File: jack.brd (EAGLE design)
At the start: 100 x 80 mm, 30 parts, among them IC1 NUF2221W1T2G, IC2 ATSAMD21G18, IC3 LDO, SW1 SPST3.5X6MM, X1 TSX-3225 24.0000MF10Z-C3

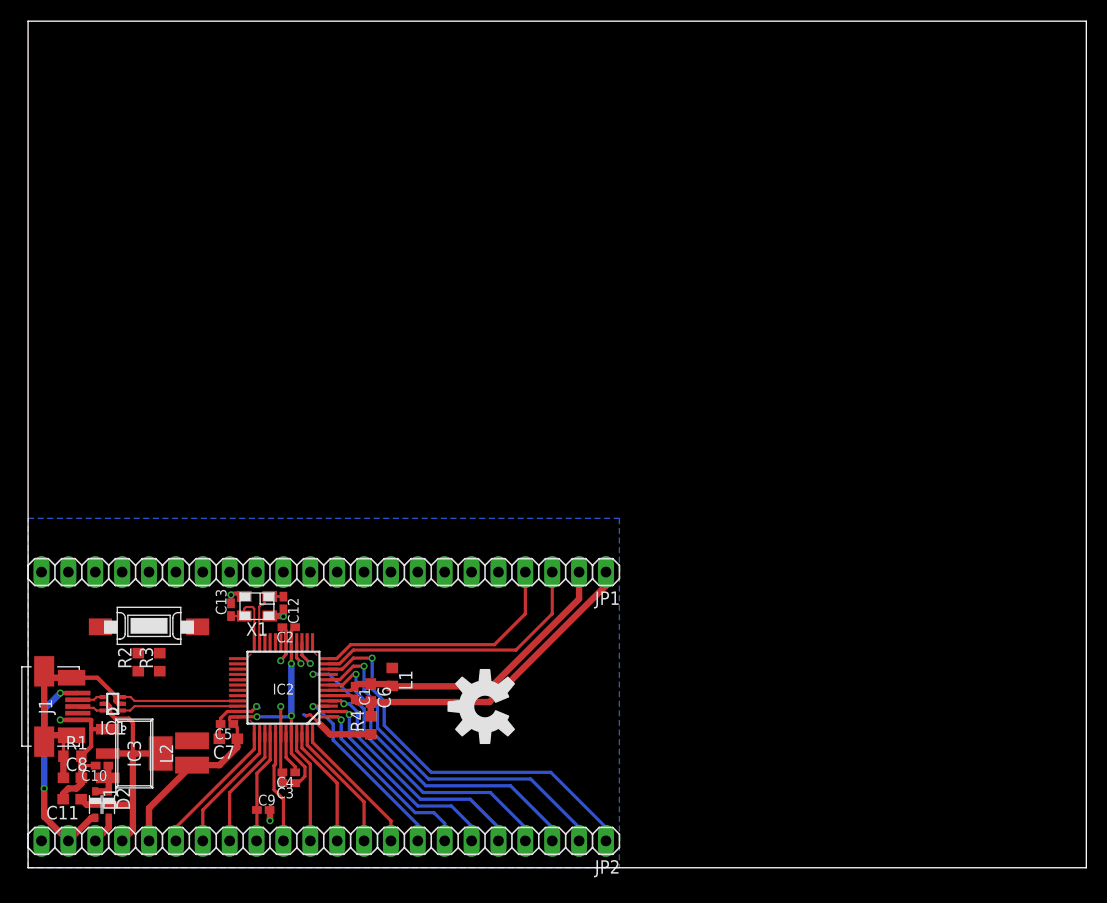
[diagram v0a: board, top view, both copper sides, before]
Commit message: :feelsgood: Layout finished!
Minor details gotta be worked now (polishing pours layout)
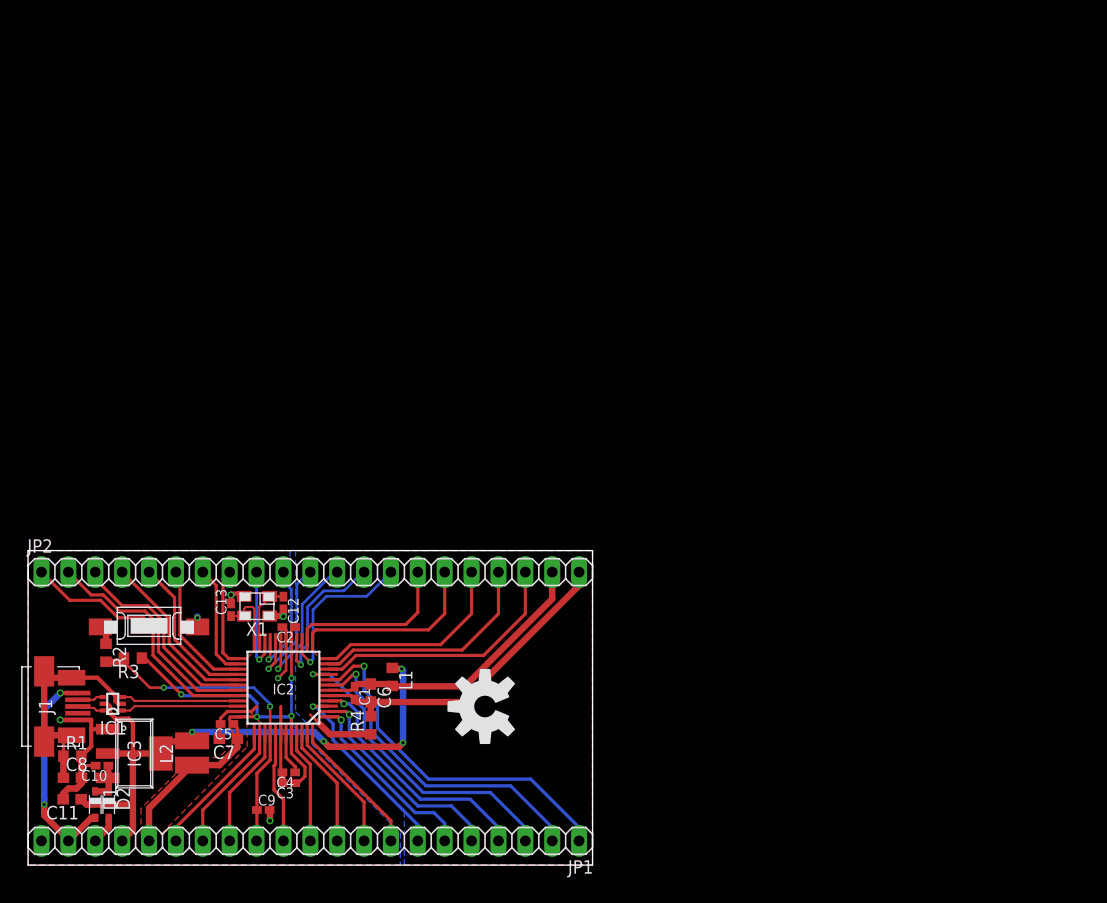
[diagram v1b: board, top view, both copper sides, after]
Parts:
- JP1, JP2: value (none) -> PINHD-1X21; device pinhead:1X22 -> jack:1X21
- moved JP1 25.4 mm to (26.7, 2.54)
- moved JP2 25.4 mm to (26.7, 27.9), turned to 0 degrees
- moved R2 3.18 mm to (7.37, 20.3), turned to 270 degrees
- moved R3 2.57 mm to (9.91, 19.8), turned to 180 degrees
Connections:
- removed net NC: JP1.10, JP1.11, JP1.12, JP1.13, JP1.14, JP1.15, JP1.16, JP1.17, JP1.18, JP1.9
- net !RESET: now also JP1.13; no longer JP2.14
- net 1: now also JP1.6; no longer JP2.7
- net 10: now also JP2.19; no longer JP2.1
- net 11: now also JP2.18; no longer JP1.3
- net 12: now also JP2.17; no longer JP1.4
- net 13: now also JP2.16; no longer JP1.5
- net 14: now also JP2.15; no longer JP1.6
- net 15: now also JP2.14; no longer JP1.7
- net 16: now also JP2.13; no longer JP1.8
- net 19: now also JP2.12; no longer JP1.19
- net 2: now also JP1.5; no longer JP2.6
- net 20: now also JP2.11; no longer JP1.20
- net 21: now also JP2.10; no longer JP1.21
- net 22: now also JP2.9; no longer JP1.22
- net 25: now also JP2.8
- net 26: now also JP2.7
- net 27: now also JP2.6
- net 28: now also JP2.5
- net 29: now also JP2.4
- net 3: now also JP1.7; no longer JP2.8
- net 30: now also JP2.3
- net 31: now also JP2.2
- net 32: now also JP2.1
- net 37: now also JP1.16; no longer JP2.17
- net 38: now also JP1.15; no longer JP2.16
- net 39: now also JP1.14; no longer JP2.15
- net 4: now also JP1.4; no longer JP2.5
- net 41: now also JP1.12; no longer JP2.13
- net 47: now also JP1.9; no longer JP2.10
- net 48: now also JP1.8; no longer JP2.9
- net 7: now also JP1.2; no longer JP2.3
- net 8: now also JP1.1; no longer JP2.2
- net 9: now also JP1.3; no longer JP2.4
- net GND: now also JP1.21; no longer JP2.22
- net GNDANA: now also JP2.21; no longer JP1.1
- net SWCLK: now also JP1.11; no longer JP2.12
- net SWDIO: now also JP1.10; no longer JP2.11
- net VBUS: now also JP1.20; no longer JP2.21
- net VDD: now also JP1.18; no longer JP2.19
- net VDDANA: now also JP2.20; no longer JP1.2
- net VDDF: now also JP1.17; no longer JP2.18
- net VIN: now also JP1.19; no longer JP2.20
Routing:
- net VDD: track 25.7 -> 59.3 mm, vias 0 -> 4
- net 32: track 0.00 -> 25.0 mm
- net 31: track 0.00 -> 22.2 mm
- net !RESET: track 10.8 -> 31.0 mm, vias 0 -> 2
- net 30: track 0.00 -> 19.7 mm
- net 13: track 0.00 -> 18.1 mm
- net 29: track 0.00 -> 16.5 mm
- net 14: track 0.00 -> 16.2 mm
- net 28: track 0.00 -> 14.8 mm
- net 19: track 0.00 -> 14.2 mm, vias 0 -> 1
- net VDDF: track 38.9 -> 52.9 mm, vias 3 -> 4
- net 15: track 2.29 -> 16.1 mm
- net 20: track 0.00 -> 13.6 mm, vias 0 -> 1
- net 27: track 0.00 -> 13.0 mm
- net 10: track 37.6 -> 24.7 mm, vias 1 -> 0
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- added copper zone on layer 16, net GNDANA
- added copper zone on layer 1, net VDDF
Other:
- board size 100 x 80 mm -> 53.3 x 29.7 mm
